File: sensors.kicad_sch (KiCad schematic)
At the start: 18 parts, among them U4 ICM42605, U5 MMC5983MA, U6 ICP20100

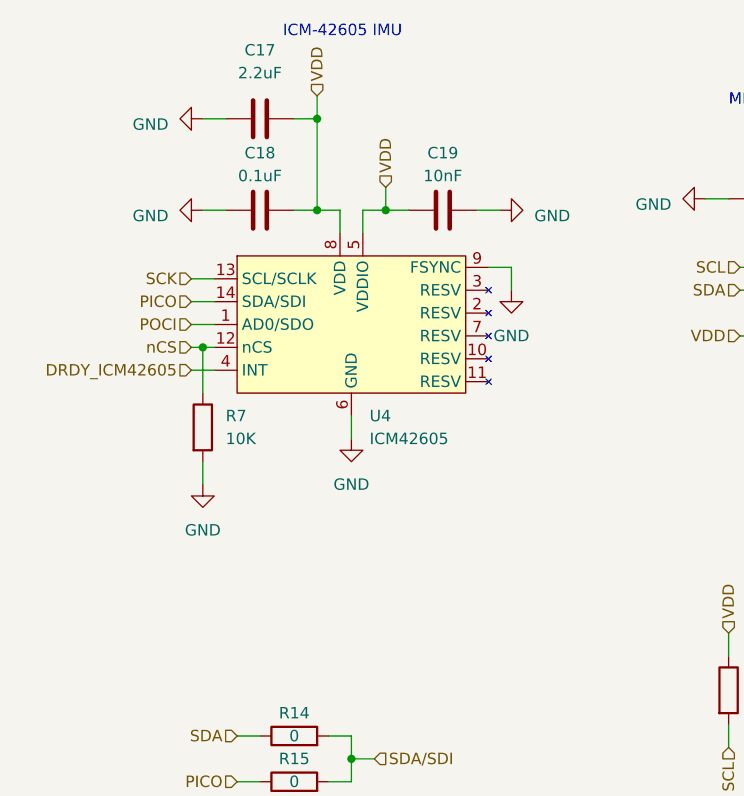
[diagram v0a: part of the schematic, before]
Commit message: Finish R01B
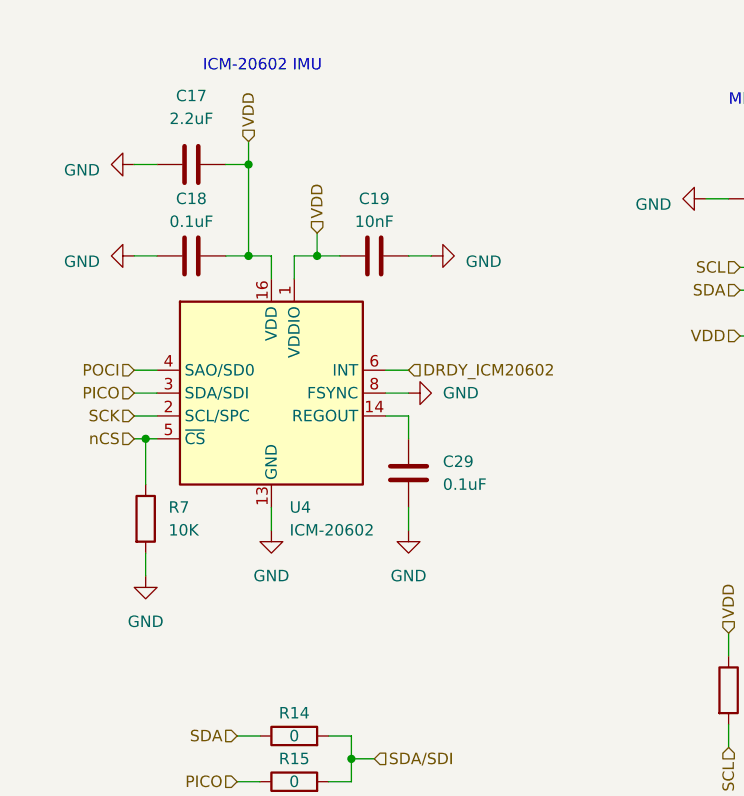
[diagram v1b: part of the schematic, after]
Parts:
- removed U4: ICM42605, Package_LGA:LGA-14_3x2.5mm_P0.5mm_LayoutBorder3x4y, symbol ICM42605:ICM42605
- added C29: 0.1uF, Capacitor_SMD:C_0402_1005Metric, symbol Device:C
- added U4: ICM-20602, Package_LGA:LGA-16_3x3mm_P0.5mm_LayoutBorder3x5y, symbol Sensor_Motion:ICM-20602
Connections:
- net GND: now also C29.2, U4.10 (GND), U4.11 (GND), U4.12 (GND), U4.13 (GND), U4.15 (GND), U4.8 (FSYNC), U4.9 (GND)
- net PICO: now also U4.3 (SDA/SDI)
- net POCI: now also U4.4 (SAO/SD0)
- net SCK: now also U4.2 (SCL/SPC)
- net VDD: now also U4.1 (VDDIO), U4.16 (VDD)
- net nCS: now also U4.5 (~{CS})
- new net: C29.1, U4.14 (REGOUT)
- new net DRDY_ICM20602: U4.6 (INT)
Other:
- note added: "ICM-20602 IMU"
- note removed: "ICM-42605 IMU"
- moved on the sheet: C17, C18, C19, R7
